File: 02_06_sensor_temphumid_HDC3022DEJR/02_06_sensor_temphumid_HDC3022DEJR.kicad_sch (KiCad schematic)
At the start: 14 parts, among them J1 MICROMOD-2222, U1 HDC3022DEJR, U2 AP2112K-3.3

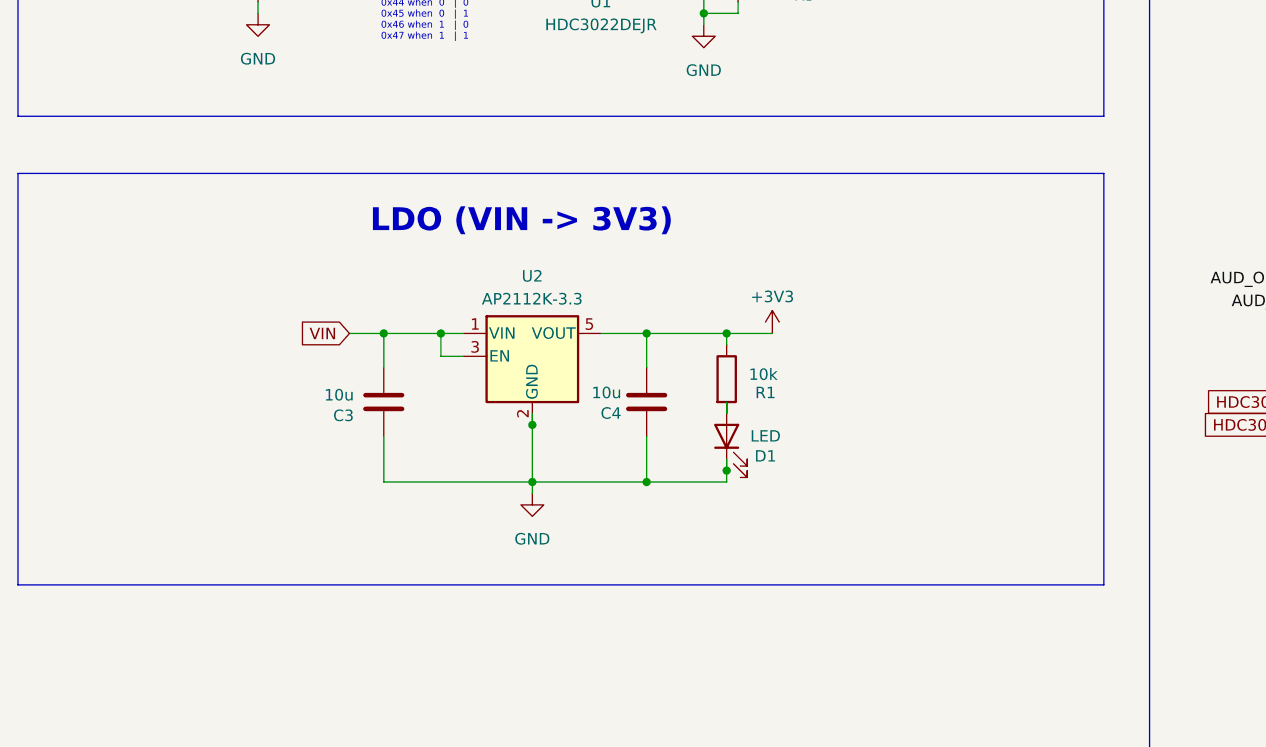
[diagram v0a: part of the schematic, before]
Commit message: filled missing connections :/
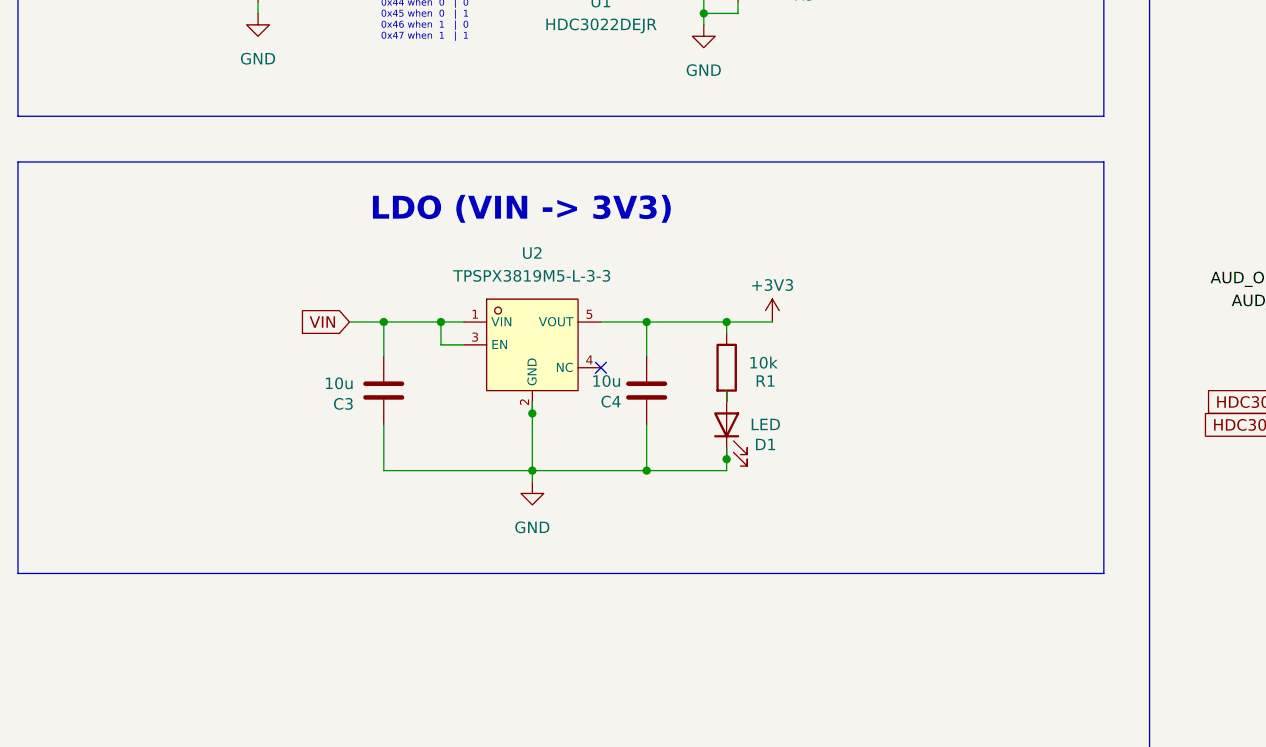
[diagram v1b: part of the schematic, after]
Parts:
- removed U2: AP2112K-3.3, Package_TO_SOT_SMD:SOT-23-5, symbol Regulator_Linear:AP2112K-3.3
- added U2: TPSPX3819M5-L-3-3, TPSPX3819M5-L-3-3:SOT-23-5_L3.0-W1.6-P0.95-LS2.8-BR, symbol TPSPX3819M5-L-3-3:TPSPX3819M5-L-3-3
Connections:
- net +3V3: now also U2.5 (VOUT)
- net GND: now also U2.2 (GND)
- net VIN: now also U2.1 (VIN), U2.3 (EN)
- no-connect marks 54 -> 55
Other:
- moved on the sheet: C3, C4, D1, R1
